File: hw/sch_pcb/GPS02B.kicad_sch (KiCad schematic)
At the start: 64 parts, among them J1 HEADER_2x03_PARALLEL, J10 HEADER_2x01_PARALLEL, J11 HEADER_2x01_PARALLEL, J12 HEADER_2x01_PARALLEL, J13 HEADER_2x01_PARALLEL, J14 HEADER_2x01_PARALLEL, J15 HEADER_2x03_PARALLEL, J16 HEADER_2x01_PARALLEL, J18 SMA, J2 USB_B, J3 HEADER_2x03_PARALLEL, J4 HEADER_2x01_PARALLEL, J5 HEADER_2x01_PARALLEL, J6 HEADER_2x01_PARALLEL, J7 HEADER_2x01_PARALLEL, J8 HEADER_2x01_PARALLEL, J9 HEADER_2x01_PARALLEL, M1 HOLE, M2 HOLE, M3 HOLE, M4 HOLE, Q1 BC817-25, U1 USBLC6-2SC6, U2 MIC5504-3.3YM5, U3 NEO-M8P

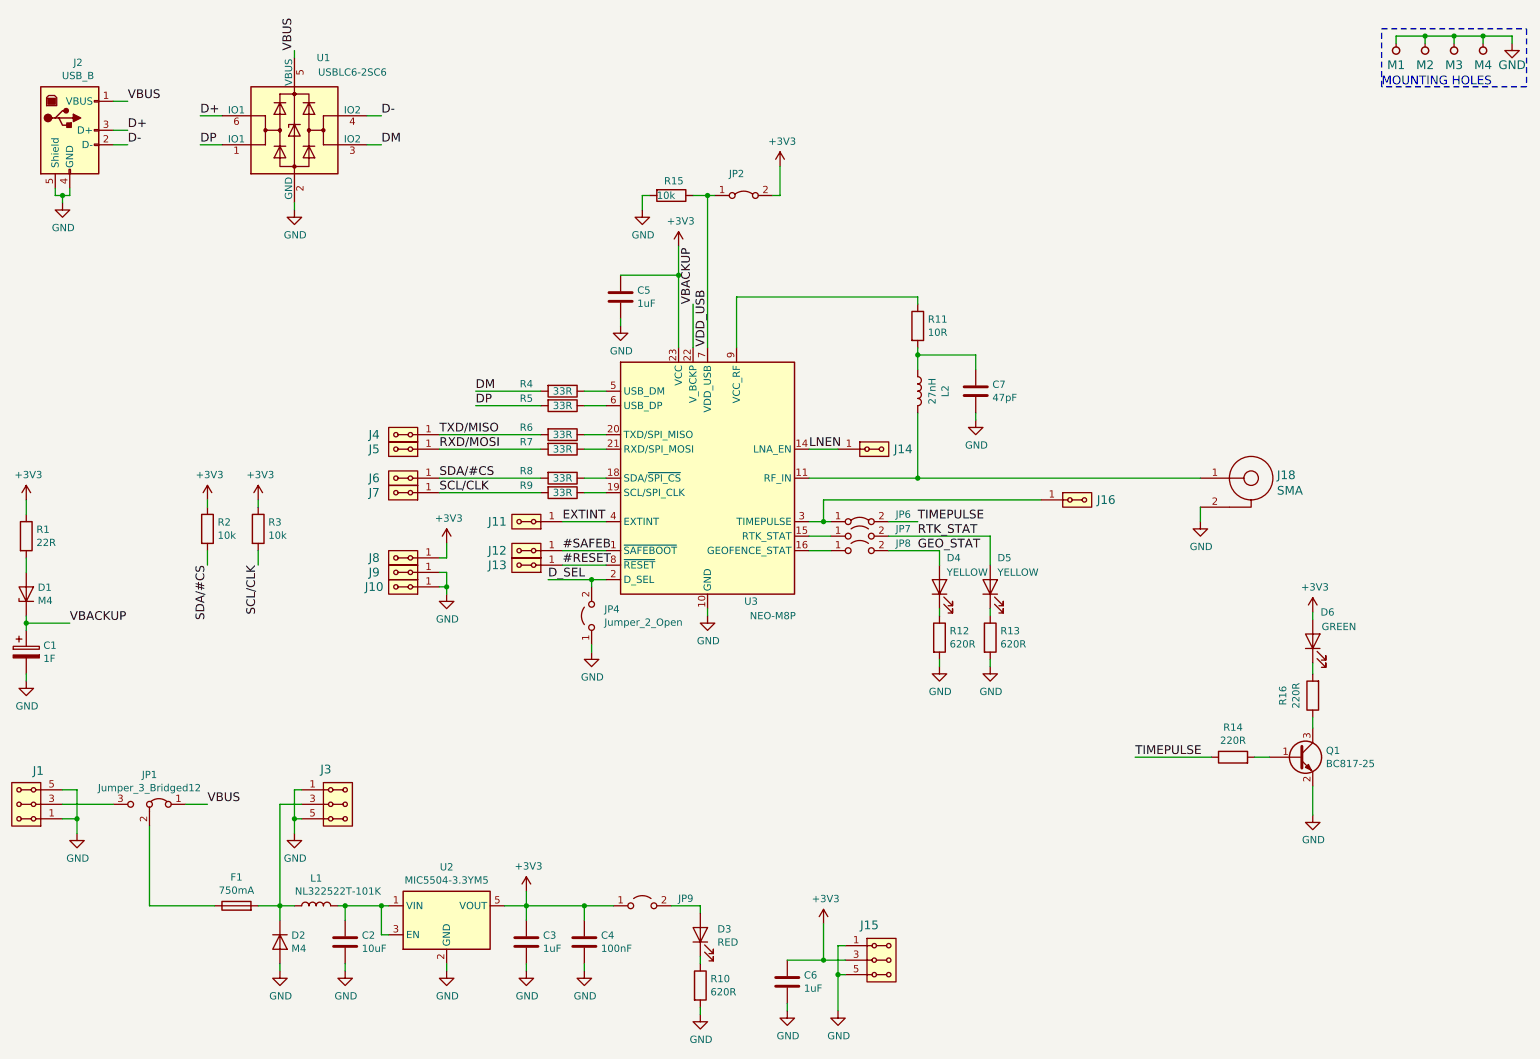
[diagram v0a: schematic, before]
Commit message: Edit bom
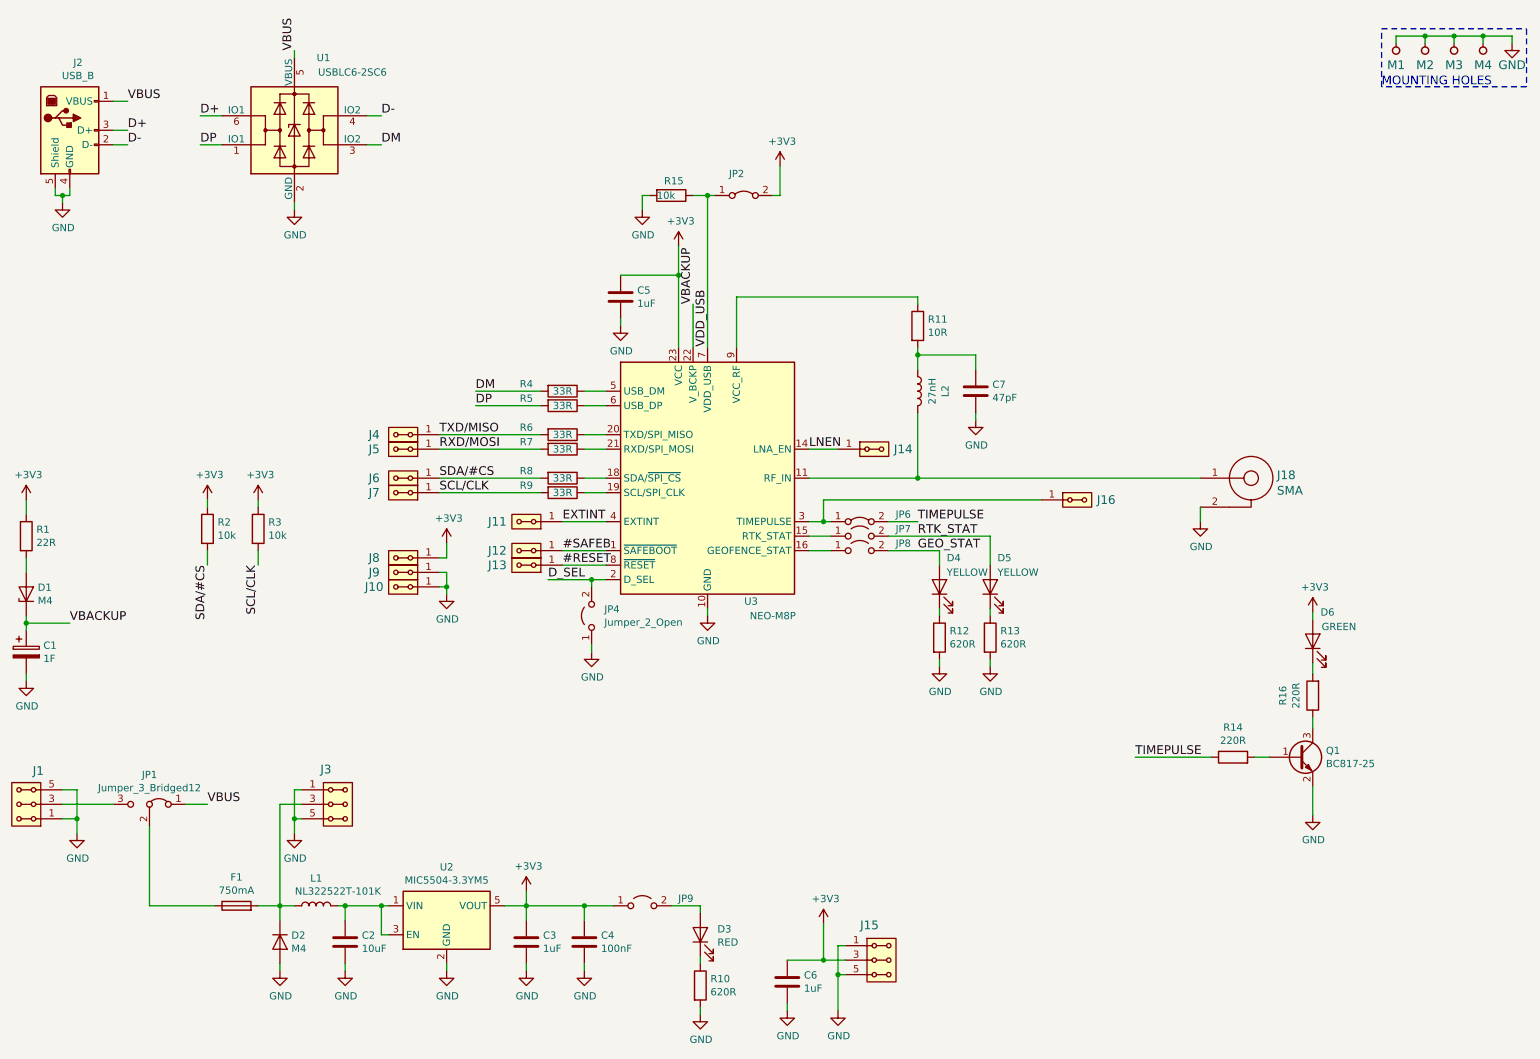
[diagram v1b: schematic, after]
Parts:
- C7: UST_ID (none) -> 5c70984712875079b91f8b38
- L2: UST_ID (none) -> 618cbf071287506e2801ed7e
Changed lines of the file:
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@@
-(kicad_sch (version 20210406) (generator eeschema)
+(kicad_sch (version 20210621) (generator eeschema)
   (paper "A4")
   (title_block
@@
       (effects (font (size 1.27 1.27)) hide)
     )
-    (property "UST_ID" "" (id 4) (at 175.26 80.01 0)
+    (property "UST_ID" "618cbf071287506e2801ed7e" (id 4) (at 175.26 80.01 0)
       (effects (font (size 1.27 1.27)) hide)
     )
@@
       (effects (font (size 1.27 1.27)) hide)
     )
-    (property "UST_ID" "" (id 4) (at 185.42 80.01 0)
-      (effects (font (size 1.27 1.27)) hide)
-    )
+    (property "UST_ID" "5c70984712875079b91f8b38" (id 4) (at 185.42 80.01 0)
+      (effects (font (size 1.27 1.27)) hide)
+    )

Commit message: Edit BOM
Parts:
- D1: UST_ID 5c70984512875079b91f88b3 -> 5c70984512875079b91f88ac
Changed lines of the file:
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@@
       (effects (font (size 1.27 1.27)) hide)
     )
-    (property "UST_ID" "5c70984512875079b91f88b3" (id 4) (at 19.05 115.57 0)
+    (property "UST_ID" "5c70984512875079b91f88ac" (id 4) (at 19.05 115.57 0)
       (effects (font (size 1.27 1.27)) hide)
     )
